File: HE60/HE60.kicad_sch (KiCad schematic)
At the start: 267 parts, among them J1 TYPE-C-31-M-12, J2 JST_SH, J3 TC2030, SW1 TS-1187A-B-A-B, SW2 TS-1187A-B-A-B, U1 STM32F446RET6, U2 USBLC6-2SC6, U3 TLV75733PDBVR, U4 TLV75733PDBVR, Y1 X322516MLB4SI

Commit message: :fire: remove op amp & update PCB
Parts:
- removed C93, C94, C95: 2.2u, Capacitor_SMD:C_0603_1608Metric, symbol Device:C
- removed H1, H2, H3, H4, H5, H6, H7, H8: SpacerHole, HE60:SpacerHole, symbol Mechanical:MountingHole
- removed HE1, HE10, HE11, HE12, HE13, HE14, HE15, HE16, HE17, HE18, HE19, HE2, HE20, HE21, HE22, HE23, HE24, HE25, HE26, HE27, HE28, HE29, HE3, HE30, HE31, HE32, HE33, HE34, HE35, HE36, HE37, HE38, HE39, HE4, HE40, HE41, HE42, HE43, HE44, HE45, HE46, HE47, HE48, HE49, HE5, HE50, HE51, HE52, HE53, HE54, HE55, HE56, HE57, HE58, HE59, HE6, HE60, HE61, HE62, HE63, HE64, HE65, HE66, HE67, HE7, HE8, HE9: GH39F, Package_TO_SOT_SMD:SOT-23-3, symbol HE60:GH39F
- removed J2: JST_SH, Connector_JST:JST_SH_SM04B-SRSS-TB_1x04-1MP_P1.00mm_Horizontal, symbol Connector_Generic:Conn_01x04
- removed OP1, OP2, OP3: GS8094-SR, Package_SO:SOIC-14_3.9x8.7mm_P1.27mm, symbol HE60:GS8094-SR
- removed U1: STM32F446RET6, Package_QFP:LQFP-64_10x10mm_P0.5mm, symbol MCU_ST_STM32F4:STM32F446RETx
- removed U2: USBLC6-2SC6, Package_TO_SOT_SMD:SOT-23-6, symbol Power_Protection:USBLC6-2SC6
- removed U3, U4: TLV75733PDBVR, Package_TO_SOT_SMD:SOT-23-5, symbol HE60:TLV75733PDBVR
- added FB1: 100R@100MHz, Inductor_SMD:L_0805_2012Metric, symbol Device:FerriteBead
- added H1, H2, H3, H4, H5, H6, H7, H8: SpacerHole, MountingHole:MountingHole_2.2mm_M2_Pad, symbol Mechanical:MountingHole_Pad
- added HE1, HE10, HE11, HE12, HE13, HE14, HE15, HE16, HE17, HE18, HE19, HE2, HE20, HE21, HE22, HE23, HE24, HE25, HE26, HE27, HE28, HE29, HE3, HE30, HE31, HE32, HE33, HE34, HE35, HE36, HE37, HE38, HE39, HE4, HE40, HE41, HE42, HE43, HE44, HE45, HE46, HE47, HE48, HE49, HE5, HE50, HE51, HE52, HE53, HE54, HE55, HE56, HE57, HE58, HE59, HE6, HE60, HE61, HE62, HE63, HE64, HE65, HE66, HE67, HE7, HE8, HE9: OH49E-S, Package_TO_SOT_SMD:SOT-23-3, symbol HE60:OH49E-S
- added J2: JST_SH, Connector_JST:JST_SH_SM04B-SRSS-TB_1x04-1MP_P1.00mm_Horizontal, symbol Connector_Generic_MountingPin:Conn_01x04_MountingPin
- added U1: USBLC6-2SC6, Package_TO_SOT_SMD:SOT-23-6, symbol Power_Protection:USBLC6-2SC6
- added U2: TLV75733PDBV, Package_TO_SOT_SMD:SOT-23-5, symbol Regulator_Linear:TLV75733PDBV
- added U3: STM32F446RET6, Package_QFP:LQFP-64_10x10mm_P0.5mm, symbol MCU_ST_STM32F4:STM32F446RETx
- AM1, AM2, AM3, AM4, AM5, AM6, AM7, AM8, AM9: value TMUX1308PWR -> SN74LV4051A
- C77, C78: value 100n -> 2.2u; footprint Capacitor_SMD:C_0402_1005Metric -> Capacitor_SMD:C_0603_1608Metric
- C79, C80: value 100n -> 1u; footprint Capacitor_SMD:C_0402_1005Metric -> Capacitor_SMD:C_0603_1608Metric
- C85: value 10u -> 100n; footprint Capacitor_SMD:C_0603_1608Metric -> Capacitor_SMD:C_0402_1005Metric
- C86: value 100n -> 10u; footprint Capacitor_SMD:C_0402_1005Metric -> Capacitor_SMD:C_0603_1608Metric
- C87: value 1u -> 100n; footprint Capacitor_SMD:C_0603_1608Metric -> Capacitor_SMD:C_0402_1005Metric
- C88: value 4.7u -> 1u
- C89: value 10p -> 100n
- C90: value 10p -> 4.7u; footprint Capacitor_SMD:C_0402_1005Metric -> Capacitor_SMD:C_0603_1608Metric
- C91: value 100n -> 10p
- C92: value 2.2u -> 10p; footprint Capacitor_SMD:C_0603_1608Metric -> Capacitor_SMD:C_0402_1005Metric
- F1: value BSMD1206-100-16V -> BSMD0805-050-24V; footprint Fuse:Fuse_1206_3216Metric -> Fuse:Fuse_0805_2012Metric
- MX57: value 1.5 -> 1.5U
- R1: value 10k -> 5.1k
- R3: value 5.1k -> 10k
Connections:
- net +3.3V: now also C78.1, C79.1, C86.1, FB1.1, U2.5 (OUT), U3.1 (VBAT), U3.19 (VDD), U3.32 (VDD), U3.48 (VDD), U3.64 (VDD); no longer C80.1
- net +3.3VA: now also C80.1, C88.1, FB1.2, HE1.1 (VCC), HE10.1 (VCC), HE11.1 (VCC), HE12.1 (VCC), HE13.1 (VCC), HE14.1 (VCC), HE15.1 (VCC), HE16.1 (VCC), HE17.1 (VCC), HE18.1 (VCC), HE19.1 (VCC), HE2.1 (VCC), HE20.1 (VCC), HE21.1 (VCC), HE22.1 (VCC), HE23.1 (VCC), HE24.1 (VCC), HE25.1 (VCC), HE26.1 (VCC), HE27.1 (VCC), HE28.1 (VCC), HE29.1 (VCC), HE3.1 (VCC), HE30.1 (VCC), HE31.1 (VCC), HE32.1 (VCC), HE33.1 (VCC), HE34.1 (VCC), HE35.1 (VCC), HE36.1 (VCC), HE37.1 (VCC), HE38.1 (VCC), HE39.1 (VCC), HE4.1 (VCC), HE40.1 (VCC), HE41.1 (VCC), HE42.1 (VCC), HE43.1 (VCC), HE44.1 (VCC), HE45.1 (VCC), HE46.1 (VCC), HE47.1 (VCC), HE48.1 (VCC), HE49.1 (VCC), HE5.1 (VCC), HE50.1 (VCC), HE51.1 (VCC), HE52.1 (VCC), HE53.1 (VCC), HE54.1 (VCC), HE55.1 (VCC), HE56.1 (VCC), HE57.1 (VCC), HE58.1 (VCC), HE59.1 (VCC), HE6.1 (VCC), HE60.1 (VCC), HE61.1 (VCC), HE62.1 (VCC), HE63.1 (VCC), HE64.1 (VCC), HE65.1 (VCC), HE66.1 (VCC), HE67.1 (VCC), HE7.1 (VCC), HE8.1 (VCC), HE9.1 (VCC), U3.13 (VDDA); no longer C77.1, C78.1, C79.1, C86.1
- net +5V: now also C77.1, U1.5 (VBUS), U2.1 (IN), U2.3 (EN); no longer C92.1
- net BOOT0: now also R3.1, U3.60 (BOOT0); no longer R4.1
- net BOOT1: now also R4.1, U3.28 (PB2); no longer R1.1
- net GND: now also AM3.14 (X1), AM3.15 (X2), AM5.15 (X2), AM5.5 (X5), AM8.2 (X6), C89.1, C91.2, R2.1, R3.2, HE1.3 (GND), HE10.3 (GND), HE11.3 (GND), HE12.3 (GND), HE13.3 (GND), HE14.3 (GND), HE15.3 (GND), HE16.3 (GND), HE17.3 (GND), HE18.3 (GND), HE19.3 (GND), HE2.3 (GND), HE20.3 (GND), HE21.3 (GND), HE22.3 (GND), HE23.3 (GND), HE24.3 (GND), HE25.3 (GND), HE26.3 (GND), HE27.3 (GND), HE28.3 (GND), HE29.3 (GND), HE3.3 (GND), HE30.3 (GND), HE31.3 (GND), HE32.3 (GND), HE33.3 (GND), HE34.3 (GND), HE35.3 (GND), HE36.3 (GND), HE37.3 (GND), HE38.3 (GND), HE39.3 (GND), HE4.3 (GND), HE40.3 (GND), HE41.3 (GND), HE42.3 (GND), HE43.3 (GND), HE44.3 (GND), HE45.3 (GND), HE46.3 (GND), HE47.3 (GND), HE48.3 (GND), HE49.3 (GND), HE5.3 (GND), HE50.3 (GND), HE51.3 (GND), HE52.3 (GND), HE53.3 (GND), HE54.3 (GND), HE55.3 (GND), HE56.3 (GND), HE57.3 (GND), HE58.3 (GND), HE59.3 (GND), HE6.3 (GND), HE60.3 (GND), HE61.3 (GND), HE62.3 (GND), HE63.3 (GND), HE64.3 (GND), HE65.3 (GND), HE66.3 (GND), HE67.3 (GND), HE7.3 (GND), HE8.3 (GND), HE9.3 (GND), J2.4 (Pin_4), U1.2 (GND), U2.2 (GND), U3.12 (VSSA), U3.18 (VSS), U3.31 (VSS), U3.47 (VSS), U3.63 (VSS); no longer C89.2, C91.1, R2.2, R3.1
- net HE1: now also HE1.2 (OUT)
- net HE10: now also HE10.2 (OUT)
- net HE11: now also HE11.2 (OUT)
- net HE12: now also HE12.2 (OUT)
- net HE13: now also HE13.2 (OUT)
- net HE14: now also HE14.2 (OUT)
- net HE15: now also HE15.2 (OUT)
- net HE16: now also HE16.2 (OUT)
- net HE17: now also HE17.2 (OUT)
- net HE18: now also HE18.2 (OUT)
- net HE19: now also HE19.2 (OUT)
- net HE2: now also HE2.2 (OUT)
- net HE20: now also HE20.2 (OUT)
- net HE21: now also HE21.2 (OUT)
- net HE22: now also HE22.2 (OUT)
- net HE23: now also HE23.2 (OUT)
- net HE24: now also HE24.2 (OUT)
- net HE25: now also HE25.2 (OUT)
- net HE26: now also HE26.2 (OUT)
- net HE27: now also HE27.2 (OUT)
- net HE28: now also HE28.2 (OUT)
- net HE29: now also HE29.2 (OUT)
- net HE3: now also HE3.2 (OUT)
- net HE30: now also HE30.2 (OUT)
- net HE31: now also HE31.2 (OUT)
- net HE32: now also HE32.2 (OUT)
- net HE33: now also HE33.2 (OUT)
- net HE34: now also HE34.2 (OUT)
- net HE35: now also HE35.2 (OUT)
- net HE36: now also HE36.2 (OUT)
- net HE37: now also HE37.2 (OUT)
- net HE38: now also HE38.2 (OUT)
- net HE39: now also HE39.2 (OUT)
- net HE4: now also HE4.2 (OUT)
- net HE40: now also HE40.2 (OUT)
- net HE41: now also HE41.2 (OUT)
- net HE42: now also HE42.2 (OUT)
- net HE43: now also HE43.2 (OUT)
- net HE44: now also HE44.2 (OUT)
- net HE45: now also HE45.2 (OUT)
- net HE46: now also HE46.2 (OUT)
- net HE47: now also HE47.2 (OUT)
- net HE48: now also HE48.2 (OUT)
- net HE49: now also HE49.2 (OUT)
- net HE5: now also HE5.2 (OUT)
- net HE50: now also HE50.2 (OUT)
- net HE51: now also HE51.2 (OUT)
- net HE52: now also HE52.2 (OUT)
- net HE53: now also HE53.2 (OUT)
- net HE54: now also HE54.2 (OUT)
- net HE55: now also HE55.2 (OUT)
- net HE56: now also HE56.2 (OUT)
- net HE57: now also HE57.2 (OUT)
- net HE58: now also HE58.2 (OUT)
- net HE59: now also HE59.2 (OUT)
- net HE6: now also HE6.2 (OUT)
- net HE60: now also HE60.2 (OUT)
- net HE61: now also HE61.2 (OUT)
- net HE62: now also HE62.2 (OUT)
- net HE63: now also HE63.2 (OUT)
- net HE64: now also HE64.2 (OUT)
- net HE65: now also HE65.2 (OUT)
- net HE66: now also HE66.2 (OUT)
- net HE67: now also HE67.2 (OUT)
- net HE7: now also HE7.2 (OUT)
- net HE8: now also HE8.2 (OUT)
- net HE9: now also HE9.2 (OUT)
- net MUX_OUT_1: now also U3.14 (PA0)
- net MUX_OUT_2: now also U3.15 (PA1)
- net MUX_OUT_3: now also U3.16 (PA2)
- net MUX_OUT_4: now also U3.17 (PA3)
- net MUX_OUT_5: now also U3.20 (PA4)
- net MUX_OUT_6: now also U3.21 (PA5)
- net MUX_OUT_7: now also U3.22 (PA6)
- net MUX_OUT_8: now also U3.23 (PA7)
- net MUX_OUT_9: now also U3.26 (PB0)
- net MUX_SELECT_0: now also U3.2 (PC13)
- net MUX_SELECT_1: now also U3.3 (PC14)
- net MUX_SELECT_2: now also U3.4 (PC15)
- net NRST: now also C89.2, U3.7 (NRST); no longer C91.2
- net RCC_OSC_IN: now also C91.1, U3.5 (PH0); no longer C89.1
- net RCC_OSC_OUT: now also C92.1, U3.6 (PH1); no longer C90.1
- net SWCLK: now also U3.49 (PA14)
- net SWDIO: now also U3.46 (PA13)
- net SWO: now also U3.55 (PB3)
- net USB_D+: now also U1.4 (I/O2), U3.45 (PA12)
- net USB_D-: now also U1.6 (I/O1), U3.44 (PA11)
- net USB_PLUG_D+: now also J2.3 (Pin_3), U1.3 (I/O2)
- net USB_PLUG_D-: now also J2.2 (Pin_2), U1.1 (I/O1)
- net VBUS: now also J2.1 (Pin_1)
- net at J1.A5 (CC1): now also R1.1; no longer R2.1
- net at J1.B5 (CC2): now also R2.2; no longer R3.2
- new net: C90.1, U3.30 (VCAP_1)
- no-connect marks 37 -> 41
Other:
- note added: "PCB"
- note removed: "Board"
- note removed: "USB"
- note removed: "Voltage Followers"

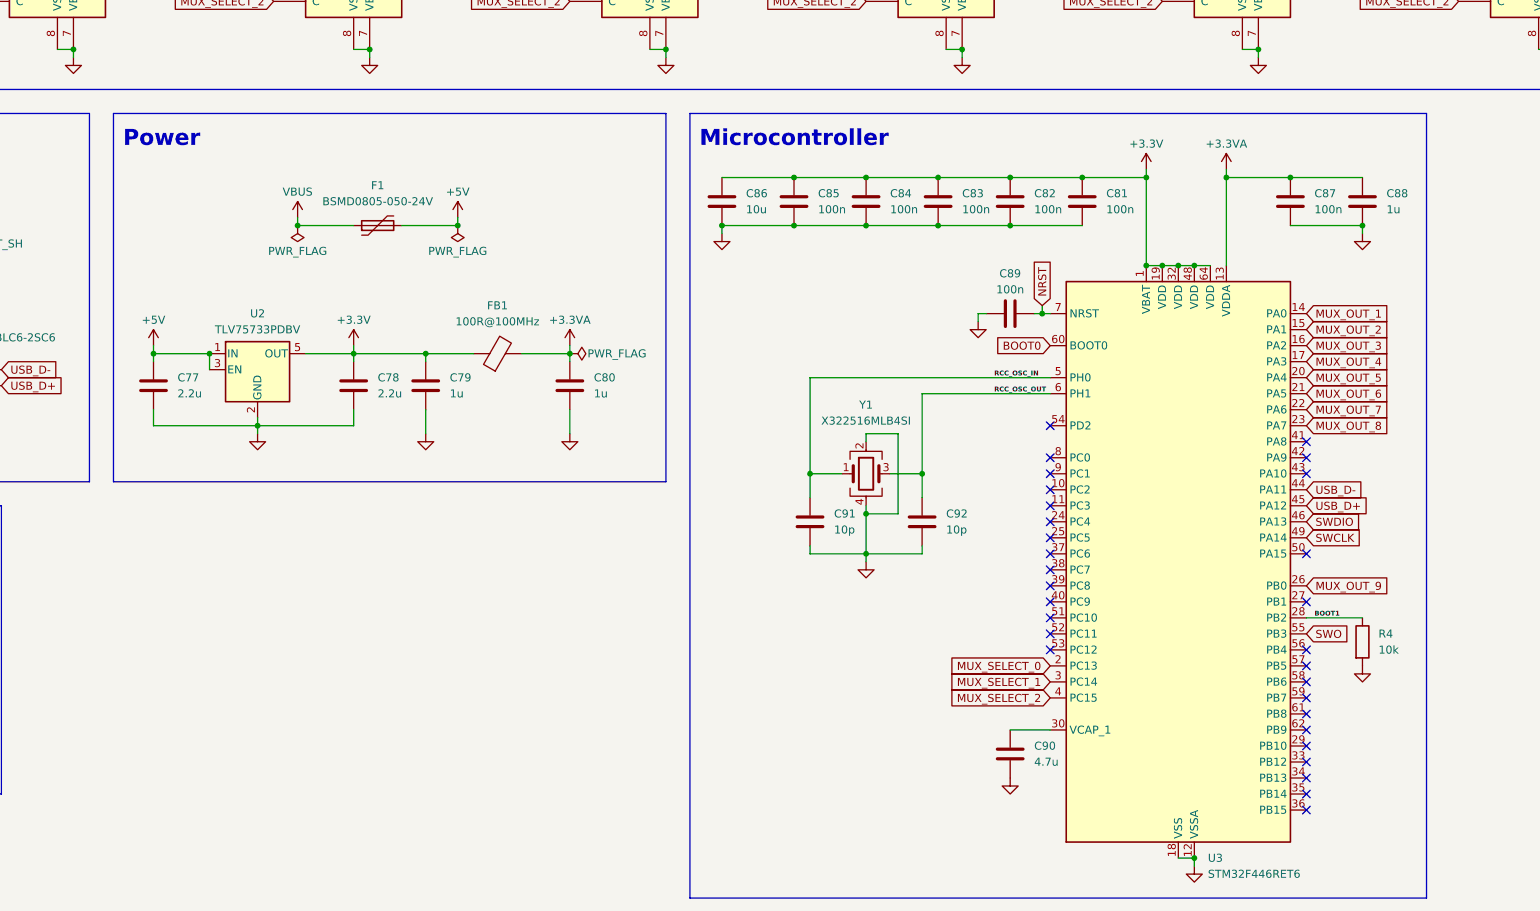
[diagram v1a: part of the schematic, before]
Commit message: :sparkles: separate voltage supplier for MCU
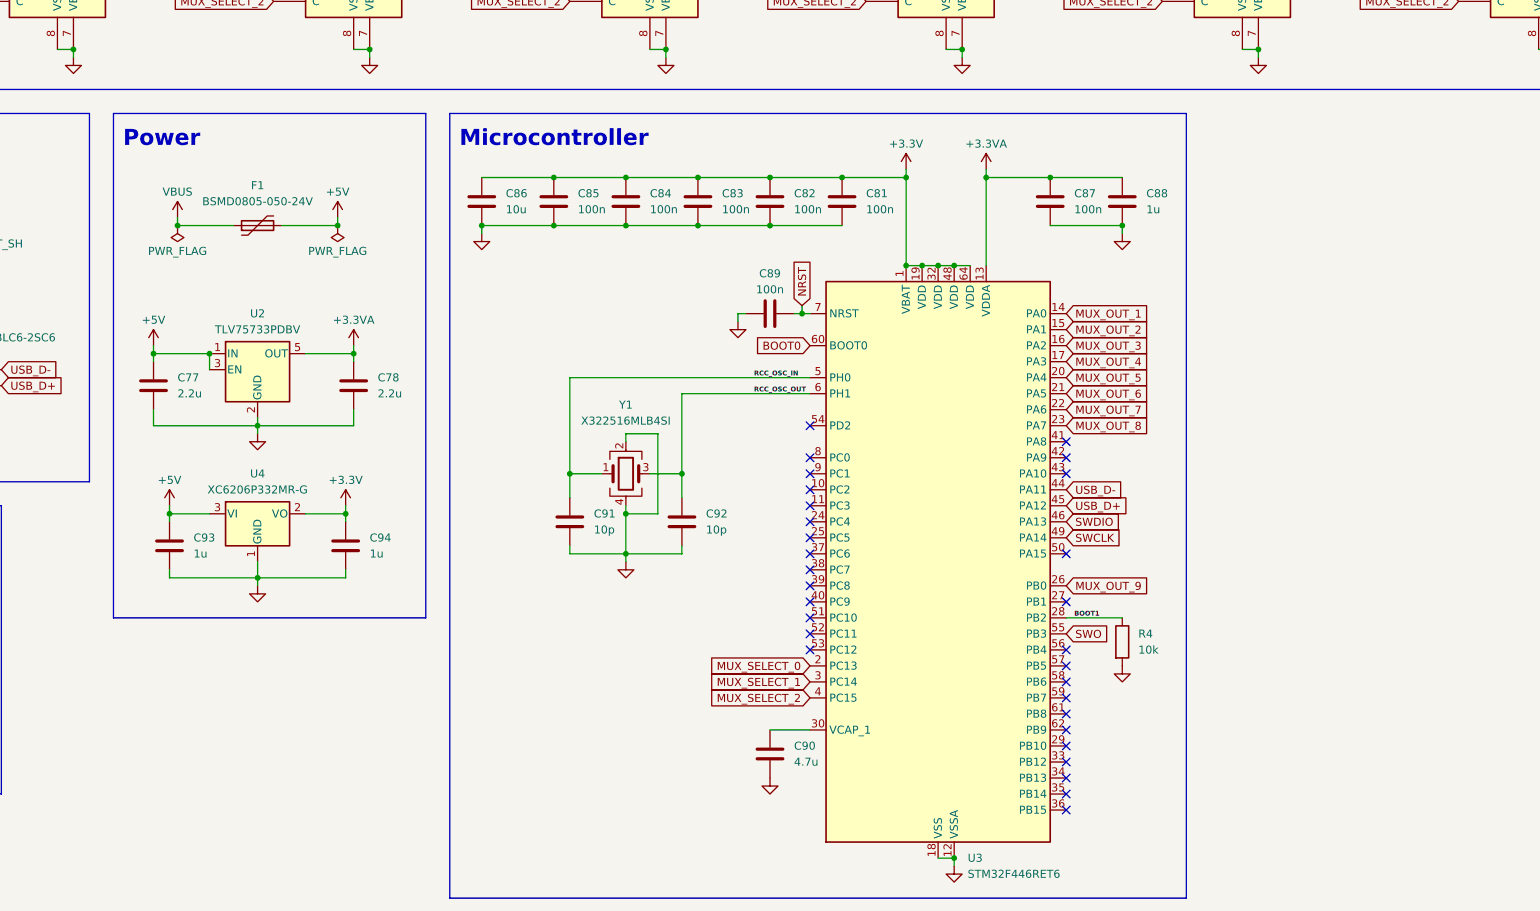
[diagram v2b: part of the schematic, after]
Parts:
- removed C79, C80: 1u, Capacitor_SMD:C_0603_1608Metric, symbol Device:C
- removed FB1: 100R@100MHz, Inductor_SMD:L_0805_2012Metric, symbol Device:FerriteBead
- added C93, C94: 1u, Capacitor_SMD:C_0603_1608Metric, symbol Device:C
- added U4: XC6206P332MR-G, Package_TO_SOT_SMD:SOT-23-3, symbol Regulator_Linear:XC6206PxxxMR
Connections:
- net +3.3V: now also C94.1, U4.2 (VO); no longer C78.1, U2.5 (OUT)
- net +3.3VA: now also C78.1, U2.5 (OUT)
- net +5V: now also C93.1, U4.3 (VI)
- net GND: now also C93.2, C94.2, U4.1 (GND)
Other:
- moved on the sheet: C81, C82, C83, C84, C85, C86, C87, C88, C89, C90, C91, C92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

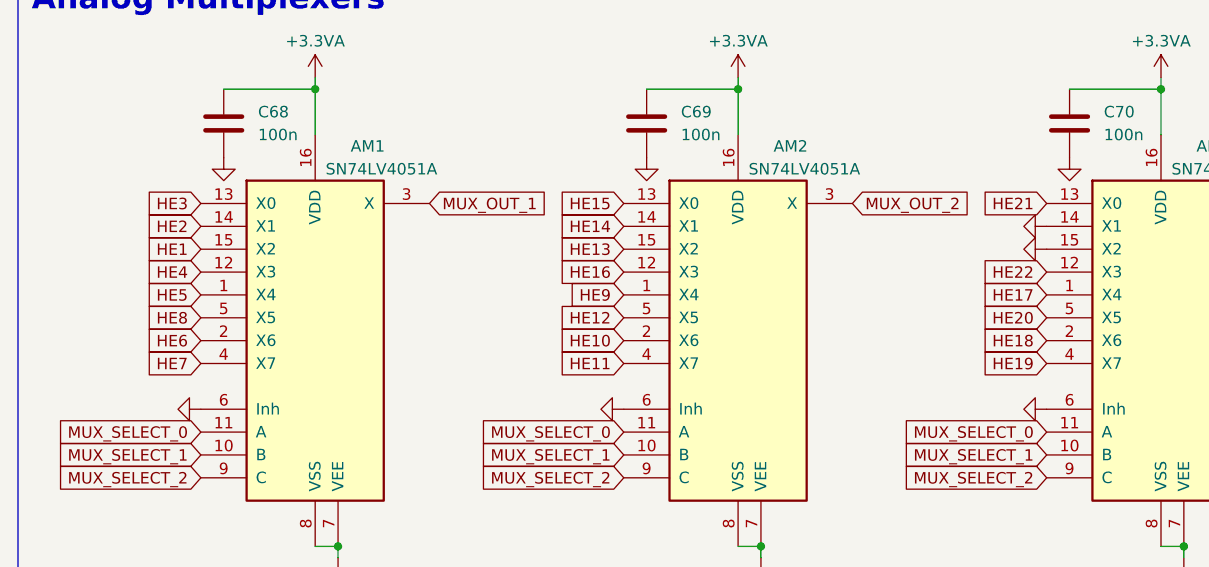
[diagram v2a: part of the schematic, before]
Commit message: :bug: fix escape key noise
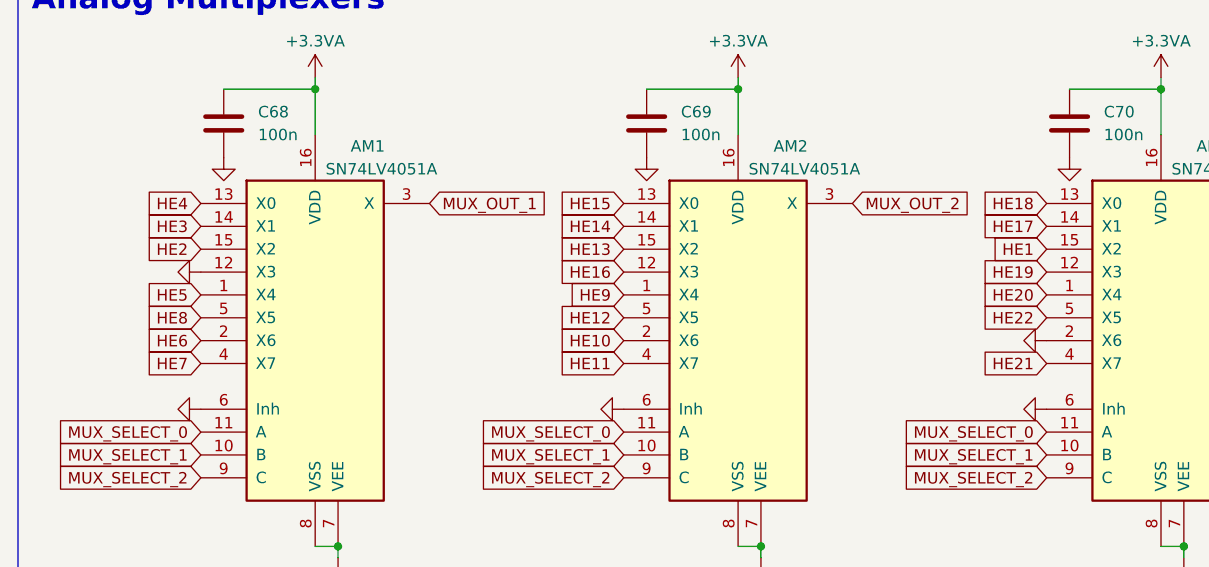
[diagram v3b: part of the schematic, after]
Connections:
- net GND: now also AM1.12 (X3), AM3.2 (X6); no longer AM3.14 (X1), AM3.15 (X2)
- net HE1: now also AM3.15 (X2); no longer AM1.15 (X2)
- net HE17: now also AM3.14 (X1); no longer AM3.1 (X4)
- net HE18: now also AM3.13 (X0); no longer AM3.2 (X6)
- net HE19: now also AM3.12 (X3); no longer AM3.4 (X7)
- net HE2: now also AM1.15 (X2); no longer AM1.14 (X1)
- net HE20: now also AM3.1 (X4); no longer AM3.5 (X5)
- net HE21: now also AM3.4 (X7); no longer AM3.13 (X0)
- net HE22: now also AM3.5 (X5); no longer AM3.12 (X3)
- net HE3: now also AM1.14 (X1); no longer AM1.13 (X0)
- net HE4: now also AM1.13 (X0); no longer AM1.12 (X3)

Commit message: :sparkles: release v2
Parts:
- removed H1, H2, H3, H4, H5, H6, H7, H8: SpacerHole, MountingHole:MountingHole_2.2mm_M2_Pad, symbol Mechanical:MountingHole_Pad
- removed HE1, HE10, HE11, HE12, HE13, HE14, HE15, HE16, HE17, HE18, HE19, HE2, HE20, HE21, HE22, HE23, HE24, HE25, HE26, HE27, HE28, HE29, HE3, HE30, HE31, HE32, HE33, HE34, HE35, HE36, HE37, HE38, HE39, HE4, HE40, HE41, HE42, HE43, HE44, HE45, HE46, HE47, HE48, HE49, HE5, HE50, HE51, HE52, HE53, HE54, HE55, HE56, HE57, HE58, HE59, HE6, HE60, HE61, HE62, HE63, HE64, HE65, HE66, HE67, HE7, HE8, HE9: OH49E-S, Package_TO_SOT_SMD:SOT-23-3, symbol HE60:OH49E-S
- removed J3: TC2030, Connector:Tag-Connect_TC2030-IDC-FP_2x03_P1.27mm_Vertical, symbol Connector:Conn_ARM_SWD_TagConnect_TC2030
- removed U3: STM32F446RET6, Package_QFP:LQFP-64_10x10mm_P0.5mm, symbol MCU_ST_STM32F4:STM32F446RETx
- removed U4: XC6206P332MR-G, Package_TO_SOT_SMD:SOT-23-3, symbol Regulator_Linear:XC6206PxxxMR
- added C100, C102, C104, C106, C108, C110, C112, C114, C116, C118, C120, C122, C124, C126, C128, C130, C132, C134, C136, C138, C80, C96, C98: 4.7n, Capacitor_SMD:C_0402_1005Metric, symbol Device:C
- added C101, C103, C105, C107, C109, C111, C113, C115, C117, C119, C121, C123, C125, C127, C129, C131, C133, C135, C137, C139, C140, C141, C142, C143, C144, C145, C146, C147, C154, C155, C156, C158, C160, C79, C95, C97, C99: 100n, Capacitor_SMD:C_0402_1005Metric, symbol Device:C
- added C148, C149, C150, C151: 2.2u, Capacitor_SMD:C_0603_1608Metric, symbol Device:C
- added C152, C153: 30p, Capacitor_SMD:C_0603_1608Metric, symbol Device:C
- added C157: 10u, Capacitor_SMD:C_0603_1608Metric, symbol Device:C
- added C159: 1u, Capacitor_SMD:C_0603_1608Metric, symbol Device:C
- added HE1, HE10, HE11, HE12, HE13, HE14, HE15, HE16, HE17, HE18, HE19, HE2, HE20, HE21, HE22, HE23, HE24, HE25, HE26, HE27, HE28, HE29, HE3, HE30, HE31, HE32, HE33, HE34, HE35, HE36, HE37, HE38, HE39, HE4, HE40, HE41, HE42, HE43, HE44, HE45, HE46, HE47, HE48, HE49, HE5, HE50, HE51, HE52, HE53, HE54, HE55, HE56, HE57, HE58, HE59, HE6, HE60, HE61, HE62, HE63, HE64, HE65, HE66, HE67, HE68, HE69, HE7, HE8, HE9: MT9102ET, Package_TO_SOT_SMD:SOT-23-3, symbol HE60:MT9102ET
- added MX68: 2.75U, HE60:MX-2.75U-ReversedStabilizers, symbol Mechanical:MountingHole
- added MX69, MX73: 1U, HE60:MX-1U, symbol Mechanical:MountingHole
- added MX70, MX72, MX74, MX76: 1.25U, HE60:MX-1.25U, symbol Mechanical:MountingHole
- added MX71, MX75: 1.5U, HE60:MX-1.5U, symbol Mechanical:MountingHole
- added U3: XC6206P332MR-G, Package_TO_SOT_SMD:SOT-23-3, symbol Regulator_Linear:XC6206PxxxMR
- added U4: AT32F405RCT7, Package_QFP:LQFP-64_10x10mm_P0.5mm, symbol HE60:AT32F405RxT7
- C10, C12, C14, C16, C18, C2, C20, C22, C24, C26, C28, C30, C32, C34, C36, C38, C4, C40, C42, C44, C46, C48, C50, C52, C54, C56, C58, C6, C60, C62, C64, C66, C68, C70, C72, C74, C76, C8, C82, C84: value 100n -> 4.7n
- C77: value 2.2u -> 100n; footprint Capacitor_SMD:C_0603_1608Metric -> Capacitor_SMD:C_0402_1005Metric
- C78: value 2.2u -> 4.7n; footprint Capacitor_SMD:C_0603_1608Metric -> Capacitor_SMD:C_0402_1005Metric
- C86: value 10u -> 4.7n; footprint Capacitor_SMD:C_0603_1608Metric -> Capacitor_SMD:C_0402_1005Metric
- C88, C94: value 1u -> 4.7n; footprint Capacitor_SMD:C_0603_1608Metric -> Capacitor_SMD:C_0402_1005Metric
- C90: value 4.7u -> 4.7n; footprint Capacitor_SMD:C_0603_1608Metric -> Capacitor_SMD:C_0402_1005Metric
- C91: value 10p -> 100n
- C92: value 10p -> 4.7n
- C93: value 1u -> 100n; footprint Capacitor_SMD:C_0603_1608Metric -> Capacitor_SMD:C_0402_1005Metric
- MX56: value 1U -> 2.75U; footprint HE60:MX-1U -> HE60:MX-2.75U
- MX57: value 1.5U -> 1U; footprint HE60:MX-1.5U -> HE60:MX-1U
- MX58, MX60: value 1U -> 1.25U; footprint HE60:MX-1U -> HE60:MX-1.25U
- MX61: value 2.25U -> 1U; footprint HE60:MX-2.25U-ReversedStabilizers -> HE60:MX-1U
- MX62: value 7U -> 1.25U; footprint HE60:MX-7U-ReversedStabilizers -> HE60:MX-1.25U
- MX63: value 2.75U -> 1.5U; footprint HE60:MX-2.75U-ReversedStabilizers -> HE60:MX-1.5U
- MX65: value 1.5U -> 2.25U; footprint HE60:MX-1.5U -> HE60:MX-2.25U-ReversedStabilizers
- MX66: value 1U -> 6.25U; footprint HE60:MX-1U -> HE60:MX-6.25U-ReversedStabilizers
- MX67: value 1.5U -> 7U; footprint HE60:MX-1.5U -> HE60:MX-7U-ReversedStabilizers
- R3, R4: value 10k -> 12k
- Y1: value X322516MLB4SI -> X322512MSB4SI
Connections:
- net BOOT1 is gone; now on net BOOT0: R4.1
- net +3.3V: now also C151.1, C154.1, C155.1, C156.1, C157.1, U3.2 (VO), U4.1 (VDD), U4.36 (VDD), U4.64 (VDD); no longer C81.1, C82.1, C83.1, C84.1, C85.1, C86.1, C94.1
- net +3.3VA: now also C77.1, C81.1, C83.1, C85.1, C89.1, C91.1, C93.1, C101.1, C103.1, C105.1, C107.1, C109.1, C111.1, C113.1, C115.1, C117.1, C119.1, C121.1, C123.1, C125.1, C127.1, C129.1, C131.1, C133.1, C135.1, C137.1, C139.1, C140.1, C141.1, C142.1, C143.1, C144.1, C145.1, C146.1, C147.1, C149.1, C158.1, C159.1, C79.1, C95.1, C97.1, C99.1, HE1.1 (VCC), HE10.1 (VCC), HE11.1 (VCC), HE12.1 (VCC), HE13.1 (VCC), HE14.1 (VCC), HE15.1 (VCC), HE16.1 (VCC), HE17.1 (VCC), HE18.1 (VCC), HE19.1 (VCC), HE2.1 (VCC), HE20.1 (VCC), HE21.1 (VCC), HE22.1 (VCC), HE23.1 (VCC), HE24.1 (VCC), HE25.1 (VCC), HE26.1 (VCC), HE27.1 (VCC), HE28.1 (VCC), HE29.1 (VCC), HE3.1 (VCC), HE30.1 (VCC), HE31.1 (VCC), HE32.1 (VCC), HE33.1 (VCC), HE34.1 (VCC), HE35.1 (VCC), HE36.1 (VCC), HE37.1 (VCC), HE38.1 (VCC), HE39.1 (VCC), HE4.1 (VCC), HE40.1 (VCC), HE41.1 (VCC), HE42.1 (VCC), HE43.1 (VCC), HE44.1 (VCC), HE45.1 (VCC), HE46.1 (VCC), HE47.1 (VCC), HE48.1 (VCC), HE49.1 (VCC), HE5.1 (VCC), HE50.1 (VCC), HE51.1 (VCC), HE52.1 (VCC), HE53.1 (VCC), HE54.1 (VCC), HE55.1 (VCC), HE56.1 (VCC), HE57.1 (VCC), HE58.1 (VCC), HE59.1 (VCC), HE6.1 (VCC), HE60.1 (VCC), HE61.1 (VCC), HE62.1 (VCC), HE63.1 (VCC), HE64.1 (VCC), HE65.1 (VCC), HE66.1 (VCC), HE67.1 (VCC), HE68.1 (VCC), HE69.1 (VCC), HE7.1 (VCC), HE8.1 (VCC), HE9.1 (VCC), U4.13 (VDDA); no longer C10.1, C12.1, C14.1, C16.1, C18.1, C2.1, C20.1, C22.1, C24.1, C26.1, C28.1, C30.1, C32.1, C34.1, C36.1, C38.1, C4.1, C40.1, C42.1, C44.1, C46.1, C48.1, C50.1, C52.1, C54.1, C56.1, C58.1, C6.1, C60.1, C62.1, C64.1, C66.1, C68.1, C70.1, C72.1, C74.1, C76.1, C78.1, C8.1, C88.1
- net +5V: now also C148.1, C150.1, U3.3 (VI); no longer C77.1, C93.1
- net BOOT0: now also U4.60 (PF11/BOOT0); no longer R3.1
- net GND: now also C89.2, R3.1, C100.2, C101.2, C102.2, C103.2, C104.2, C105.2, C106.2, C107.2, C108.2, C109.2, C110.2, C111.2, C112.2, C113.2, C114.2, C115.2, C116.2, C117.2, C118.2, C119.2, C120.2, C121.2, C122.2, C123.2, C124.2, C125.2, C126.2, C127.2, C128.2, C129.2, C130.2, C131.2, C132.2, C133.2, C134.2, C135.2, C136.2, C137.2, C138.2, C139.2, C140.2, C141.2, C142.2, C143.2, C144.2, C145.2, C146.2, C147.2, C148.2, C149.2, C150.2, C151.2, C152.2, C153.2, C154.2, C155.2, C156.2, C157.2, C158.2, C159.2, C160.2, C79.2, C80.2, C95.2, C96.2, C97.2, C98.2, C99.2, HE1.3 (GND), HE10.3 (GND), HE11.3 (GND), HE12.3 (GND), HE13.3 (GND), HE14.3 (GND), HE15.3 (GND), HE16.3 (GND), HE17.3 (GND), HE18.3 (GND), HE19.3 (GND), HE2.3 (GND), HE20.3 (GND), HE21.3 (GND), HE22.3 (GND), HE23.3 (GND), HE24.3 (GND), HE25.3 (GND), HE26.3 (GND), HE27.3 (GND), HE28.3 (GND), HE29.3 (GND), HE3.3 (GND), HE30.3 (GND), HE31.3 (GND), HE32.3 (GND), HE33.3 (GND), HE34.3 (GND), HE35.3 (GND), HE36.3 (GND), HE37.3 (GND), HE38.3 (GND), HE39.3 (GND), HE4.3 (GND), HE40.3 (GND), HE41.3 (GND), HE42.3 (GND), HE43.3 (GND), HE44.3 (GND), HE45.3 (GND), HE46.3 (GND), HE47.3 (GND), HE48.3 (GND), HE49.3 (GND), HE5.3 (GND), HE50.3 (GND), HE51.3 (GND), HE52.3 (GND), HE53.3 (GND), HE54.3 (GND), HE55.3 (GND), HE56.3 (GND), HE57.3 (GND), HE58.3 (GND), HE59.3 (GND), HE6.3 (GND), HE60.3 (GND), HE61.3 (GND), HE62.3 (GND), HE63.3 (GND), HE64.3 (GND), HE65.3 (GND), HE66.3 (GND), HE67.3 (GND), HE68.3 (GND), HE69.3 (GND), HE7.3 (GND), HE8.3 (GND), HE9.3 (GND), U3.1 (GND), U4.12 (VSSA), U4.31 (VSS), U4.63 (VSS); no longer AM5.5 (X5), AM8.2 (X6), C89.1, R3.2
- net HE1: now also C2.1, HE1.2 (OUT)
- net HE10: now also C20.1, HE10.2 (OUT)
- net HE11: now also C22.1, HE11.2 (OUT)
- net HE12: now also C24.1, HE12.2 (OUT)
- net HE13: now also C26.1, HE13.2 (OUT)
- net HE14: now also C28.1, HE14.2 (OUT)
- net HE15: now also C30.1, HE15.2 (OUT)
- net HE16: now also C32.1, HE16.2 (OUT)
- net HE17: now also C34.1, HE17.2 (OUT)
- net HE18: now also C36.1, HE18.2 (OUT)
- net HE19: now also C38.1, HE19.2 (OUT)
- net HE2: now also C4.1, HE2.2 (OUT)
- net HE20: now also C40.1, HE20.2 (OUT)
- net HE21: now also C42.1, HE21.2 (OUT)
- net HE22: now also C44.1, HE22.2 (OUT)
- net HE23: now also C46.1, HE23.2 (OUT)
- net HE24: now also C48.1, HE24.2 (OUT)
- net HE25: now also C50.1, HE25.2 (OUT)
- net HE26: now also C52.1, HE26.2 (OUT)
- net HE27: now also C54.1, HE27.2 (OUT)
- net HE28: now also C56.1, HE28.2 (OUT)
- net HE29: now also C58.1, HE29.2 (OUT)
- net HE3: now also C6.1, HE3.2 (OUT)
- net HE30: now also C60.1, HE30.2 (OUT)
- net HE31: now also C62.1, HE31.2 (OUT)
- net HE32: now also C64.1, HE32.2 (OUT)
- net HE33: now also C66.1, HE33.2 (OUT)
- net HE34: now also C68.1, HE34.2 (OUT)
- net HE35: now also AM5.5 (X5), C70.1, HE35.2 (OUT); no longer AM5.14 (X1)
- net HE36: now also AM5.14 (X1), C72.1, HE36.2 (OUT); no longer AM5.13 (X0)
- net HE37: now also AM5.13 (X0), C74.1, HE37.2 (OUT); no longer AM5.12 (X3)
- net HE38: now also AM5.12 (X3), C76.1, HE38.2 (OUT); no longer AM6.1 (X4)
- net HE39: now also AM6.1 (X4), C78.1, HE39.2 (OUT); no longer AM6.2 (X6)
- net HE4: now also C8.1, HE4.2 (OUT)
- net HE40: now also AM6.2 (X6), C80.1, HE40.2 (OUT); no longer AM6.4 (X7)
- net HE41: now also AM6.4 (X7), C82.1, HE41.2 (OUT); no longer AM6.5 (X5)
- net HE42: now also AM6.5 (X5), C84.1, HE42.2 (OUT); no longer AM6.15 (X2)
- net HE43: now also AM6.15 (X2), C86.1, HE43.2 (OUT); no longer AM6.14 (X1)
- net HE44: now also C88.1, HE44.2 (OUT)
- net HE45: now also C90.1, HE45.2 (OUT)
- net HE46: now also C92.1, HE46.2 (OUT)
- net HE47: now also C94.1, HE47.2 (OUT)
- net HE48: now also AM8.2 (X6), C96.1, HE48.2 (OUT); no longer AM8.4 (X7)
- net HE49: now also AM8.4 (X7), C98.1, HE49.2 (OUT); no longer AM8.5 (X5)
- net HE5: now also C10.1, HE5.2 (OUT)
- net HE50: now also AM8.5 (X5), C100.1, HE50.2 (OUT); no longer AM9.1 (X4)
- net HE51: now also AM9.1 (X4), C102.1, HE51.2 (OUT); no longer AM9.2 (X6)
- net HE52: now also AM9.2 (X6), C104.1, HE52.2 (OUT); no longer AM9.4 (X7)
- net HE53: now also AM9.4 (X7), C106.1, HE53.2 (OUT); no longer AM9.5 (X5)
- net HE54: now also AM9.5 (X5), C108.1, HE54.2 (OUT); no longer AM9.15 (X2)
- net HE55: now also C110.1, HE55.2 (OUT)
- net HE56: now also C112.1, HE56.2 (OUT)
- net HE57: now also AM6.14 (X1), C114.1, HE57.2 (OUT); no longer AM7.15 (X2)
- net HE58: now also AM7.15 (X2), C116.1, HE58.2 (OUT); no longer AM7.14 (X1)
- net HE59: now also AM7.14 (X1), C118.1, HE59.2 (OUT); no longer AM7.13 (X0)
- net HE6: now also C12.1, HE6.2 (OUT)
- net HE60: now also AM7.13 (X0), C120.1, HE60.2 (OUT); no longer AM7.12 (X3)
- net HE61: now also AM7.12 (X3), C122.1, HE61.2 (OUT); no longer AM8.12 (X3)
- net HE62: now also AM8.12 (X3), C124.1, HE62.2 (OUT); no longer AM8.13 (X0)
- net HE63: now also AM8.13 (X0), C126.1, HE63.2 (OUT); no longer AM8.14 (X1)
- net HE64: now also AM8.14 (X1), C128.1, HE64.2 (OUT); no longer AM8.15 (X2)
- net HE65: now also AM8.15 (X2), C130.1, HE65.2 (OUT); no longer AM9.12 (X3)
- net HE66: now also AM9.12 (X3), C132.1, HE66.2 (OUT); no longer AM9.13 (X0)
- net HE67: now also AM9.13 (X0), C134.1, HE67.2 (OUT); no longer AM9.14 (X1)
- net HE7: now also C14.1, HE7.2 (OUT)
- net HE8: now also C16.1, HE8.2 (OUT)
- net HE9: now also C18.1, HE9.2 (OUT)
- net MUX_OUT_1: now also U4.17 (PA3)
- net MUX_OUT_2: now also U4.20 (PA4)
- net MUX_OUT_3: now also U4.21 (PA5)
- net MUX_OUT_4: now also U4.22 (PA6)
- net MUX_OUT_5: now also U4.23 (PA7)
- net MUX_OUT_6: now also U4.24 (PC4)
- net MUX_OUT_7: now also U4.25 (PC5)
- net MUX_OUT_8: now also U4.26 (PB0)
- net MUX_OUT_9: now also U4.27 (PB1)
- net MUX_SELECT_0: now also U4.9 (PC1)
- net MUX_SELECT_1: now also U4.10 (PC2)
- net MUX_SELECT_2: now also U4.11 (PC3)
- net NRST: now also C160.1, U4.7 (NRST); no longer C89.2
- net USB_D+: now also U4.35 (OTGHS1_D+)
- net USB_D-: now also U4.34 (OTGHS1_D-)
- net RCC_OSC_IN renamed HEXT_IN
- net HEXT_IN: now also C152.1, U4.5 (PF0/HEXT_IN); no longer C91.1
- net RCC_OSC_OUT renamed HEXT_OUT
- net HEXT_OUT: now also C153.1, U4.6 (PF1/HEXT_OUT); no longer C92.1
- new net: R3.2, U4.33 (OTGHS1_R)
- new net HE68: AM9.14 (X1), C136.1, HE68.2 (OUT)
- new net HE69: AM9.15 (X2), C138.1, HE69.2 (OUT)
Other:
- note removed: "Analog Multiplexers"
- note removed: "Debug"
- note removed: "Hall Sensors"
- note removed: "Microcontroller"
- note removed: "PCB"
- note removed: "Power"
- note removed: "Switches"
